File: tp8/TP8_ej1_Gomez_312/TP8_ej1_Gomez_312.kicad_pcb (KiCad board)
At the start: 2 copper layers, 40 x 25 mm, 14 parts, among them J1 Output - RL, J2 Input, J3 Input, J4 GND, J6 Vbase, Q1 BC548

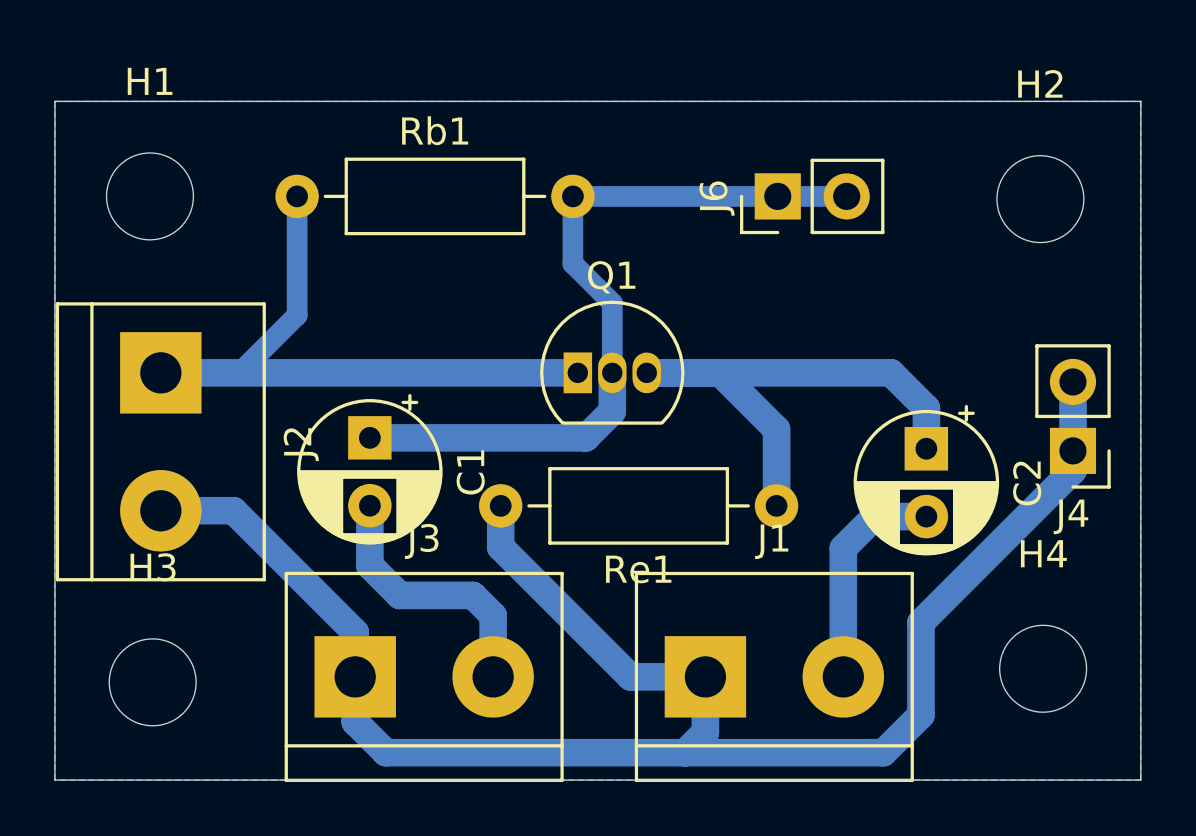
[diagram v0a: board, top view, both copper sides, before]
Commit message: finish tp8
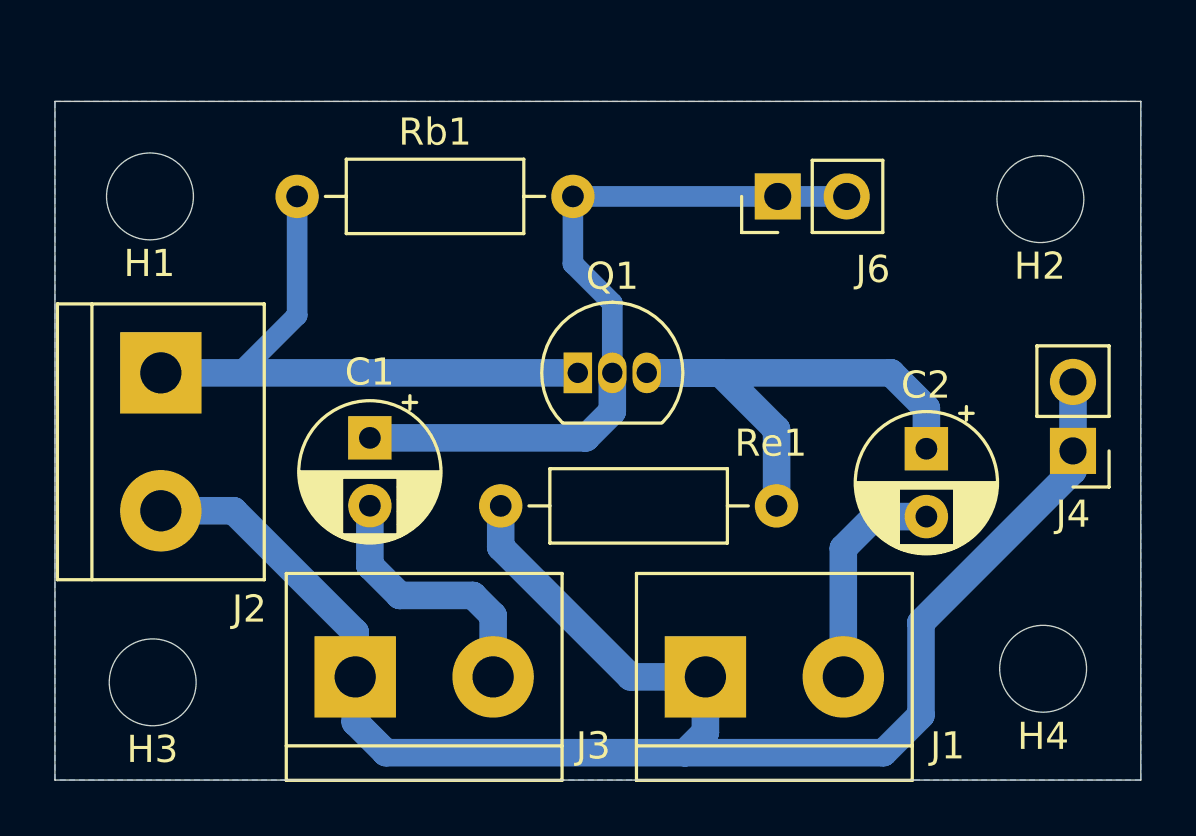
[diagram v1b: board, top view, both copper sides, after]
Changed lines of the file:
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@@
 		(tags "mounting hole 3.2mm no annular m3")
 		(property "Reference" "H1"
-			(at 0 -4.2 0)
+			(at -0.02 2.47 0)
 			(layer "F.SilkS")
 			(effects
@@
 		(tags "terminal block bornier2")
 		(property "Reference" "J3"
-			(at 2.54 -5.08 360)
+			(at 8.77 2.54 0)
 			(layer "F.SilkS")
 			(effects
@@
 		)
 		(property "Value" "Input"
-			(at 2.54 5.08 360)
+			(at 2.54 5.08 0)
 			(layer "F.Fab")
 			(effects
@@
 		)
 		(fp_text user "${REFERENCE}"
-			(at 2.54 0 360)
+			(at 2.54 0 0)
 			(layer "F.Fab")
 			(effects
@@
 		(tags "terminal block bornier2")
 		(property "Reference" "J2"
-			(at 2.54 -5.08 90)
+			(at 8.7 -3.26 180)
 			(layer "F.SilkS")
 			(effects
@@
 		(tags "terminal block bornier2")
 		(property "Reference" "J1"
-			(at 2.54 -5.08 360)
+			(at 8.92 2.54 0)
 			(layer "F.SilkS")
 			(effects
@@
 		)
 		(property "Value" "Output - RL"
-			(at 2.54 5.08 360)
+			(at 2.54 5.08 0)
 			(layer "F.Fab")
 			(effects
@@
 		)
 		(fp_text user "${REFERENCE}"
-			(at 2.54 0 360)
+			(at 2.54 0 0)
 			(layer "F.Fab")
 			(effects
@@
 		(tags "CP Radial series Radial pin pitch 2.50mm  diameter 5mm Electrolytic Capacitor")
 		(property "Reference" "C2"
-			(at 1.25 -3.75 90)
+			(at -2.344888 0.02 180)
 			(layer "F.SilkS")
 			(effects
@@
 		(tags "Through hole pin header THT 1x02 2.54mm single row")
 		(property "Reference" "J6"
-			(at 0 -2.33 270)
+			(at -2.69 3.505 0)
 			(layer "F.SilkS")
 			(effects
@@
 		)
 		(property "Value" "Vbase"
-			(at 0 4.87 270)
+			(at 0 4.87 -90)
 			(layer "F.Fab")
 			(effects
@@
 		)
 		(fp_text user "${REFERENCE}"
-			(at 0 1.27 360)
+			(at 0 1.27 0)
 			(layer "F.Fab")
 			(effects
@@
 		)
 		(fp_text user "${REFERENCE}"
-			(at 0 1.27 270)
+			(at 0 1.27 -90)
 			(layer "F.Fab")
 			(effects
@@
 		(tags "Resistor Axial_DIN0207 series Axial Horizontal pin pitch 10.16mm 0.25W = 1/4W length 6.3mm diameter 2.5mm")
 		(property "Reference" "Re1"
-			(at 5.08 -2.37 180)
+			(at 0.21 2.31 180)
 			(layer "F.SilkS")
 			(effects
@@
 		(tags "mounting hole 3.2mm no annular m3")
 		(property "Reference" "H2"
-			(at 0 -4.2 0)
+			(at -0.02 2.47 0)
 			(layer "F.SilkS")
 			(effects
@@
 		(tags "mounting hole 3.2mm no annular m3")
 		(property "Reference" "H3"
-			(at 0 -4.2 0)
+			(at -0.01 2.47 0)
 			(layer "F.SilkS")
 			(effects
@@
 		(tags "CP Radial series Radial pin pitch 2.50mm  diameter 5mm Electrolytic Capacitor")
 		(property "Reference" "C1"
-			(at 1.25 -3.75 90)
+			(at -2.424888 0.01 180)
 			(layer "F.SilkS")
 			(effects
@@
 		(tags "Resistor Axial_DIN0207 series Axial Horizontal pin pitch 10.16mm 0.25W = 1/4W length 6.3mm diameter 2.5mm")
 		(property "Reference" "Rb1"
-			(at 5.08 -2.37 360)
+			(at 5.08 -2.37 0)
 			(layer "F.SilkS")
 			(effects
@@
 		)
 		(property "Value" "1Meg"
-			(at 5.08 2.37 360)
+			(at 5.08 2.37 0)
 			(layer "F.Fab")
 			(effects
@@
 		)
 		(fp_text user "${REFERENCE}"
-			(at 5.08 0 360)
+			(at 5.08 0 0)
 			(layer "F.Fab")
 			(effects
@@
 		(tags "mounting hole 3.2mm no annular m3")
 		(property "Reference" "H4"
-			(at 0 -4.2 0)
+			(at 0 2.49 0)
 			(layer "F.SilkS")
 			(effects
@@
 		(tags "to-92 sc-43 sc-43a sot54 PA33 transistor")
 		(property "Reference" "Q1"
-			(at 1.27 -3.56 360)
+			(at 1.27 -3.56 0)
 			(layer "F.SilkS")
 			(effects
@@
 		)
 		(property "Value" "BC548"
-			(at 1.27 2.79 360)
+			(at 1.27 2.79 0)
 			(layer "F.Fab")
 			(effects
@@
 		)
 		(fp_text user "${REFERENCE}"
-			(at 1.27 0 360)
+			(at 1.27 0 0)
 			(layer "F.Fab")
 			(effects
